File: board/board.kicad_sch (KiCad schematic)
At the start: 1 part, among them U1 ESP32-S3-DevKitC

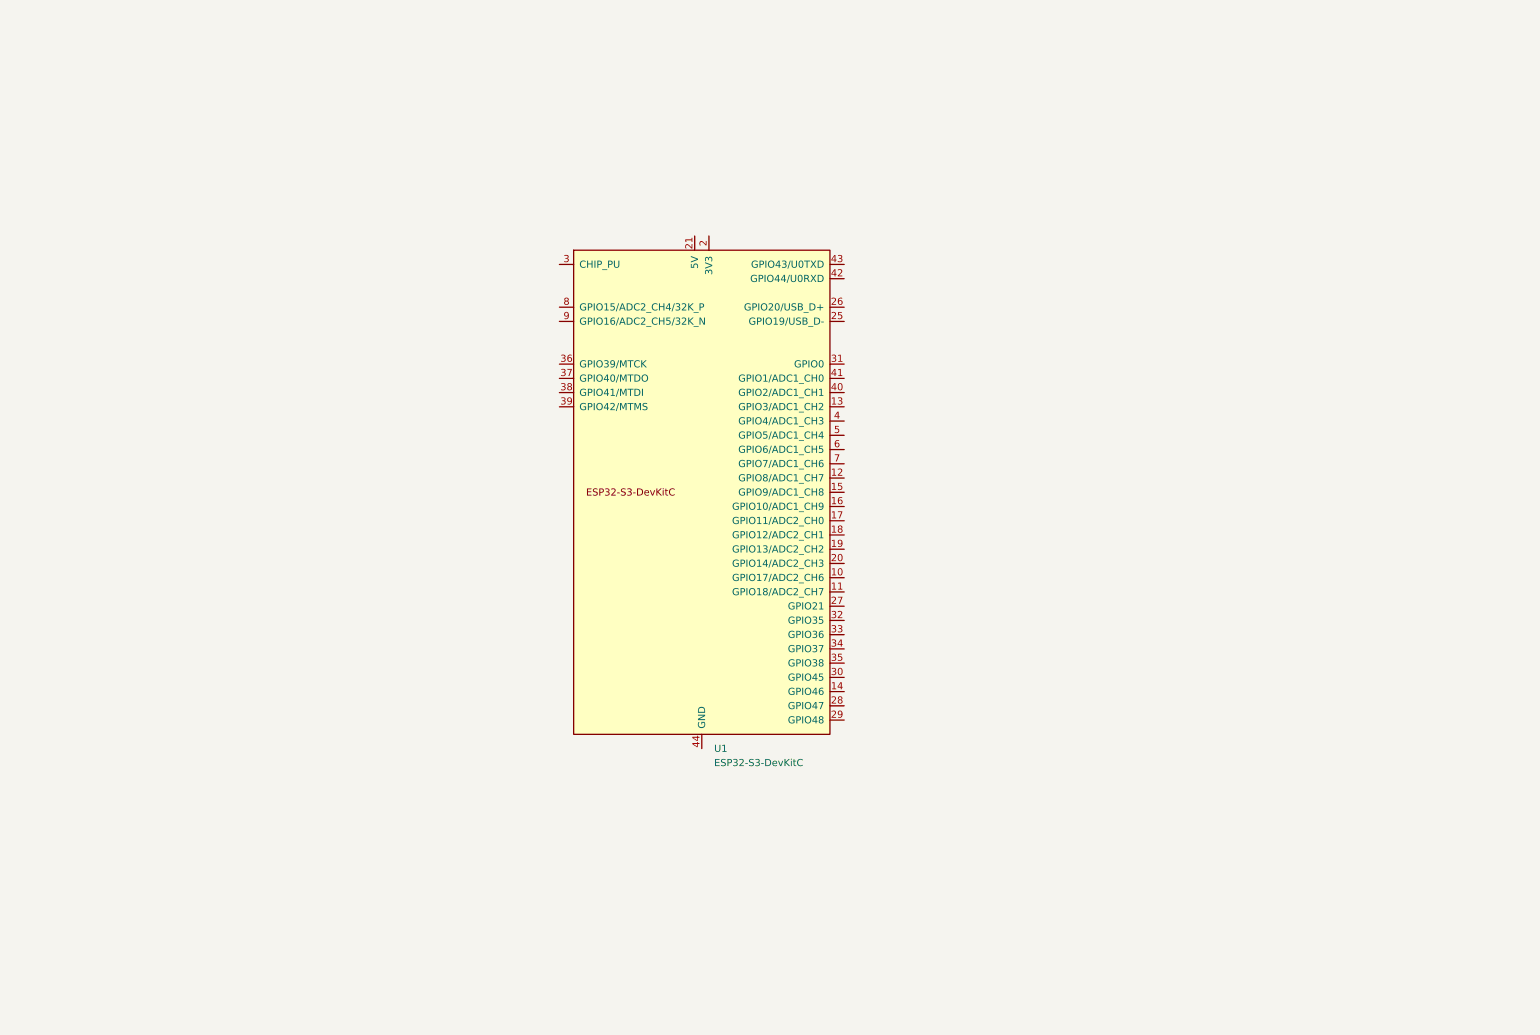
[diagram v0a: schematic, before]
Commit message: incremental changes
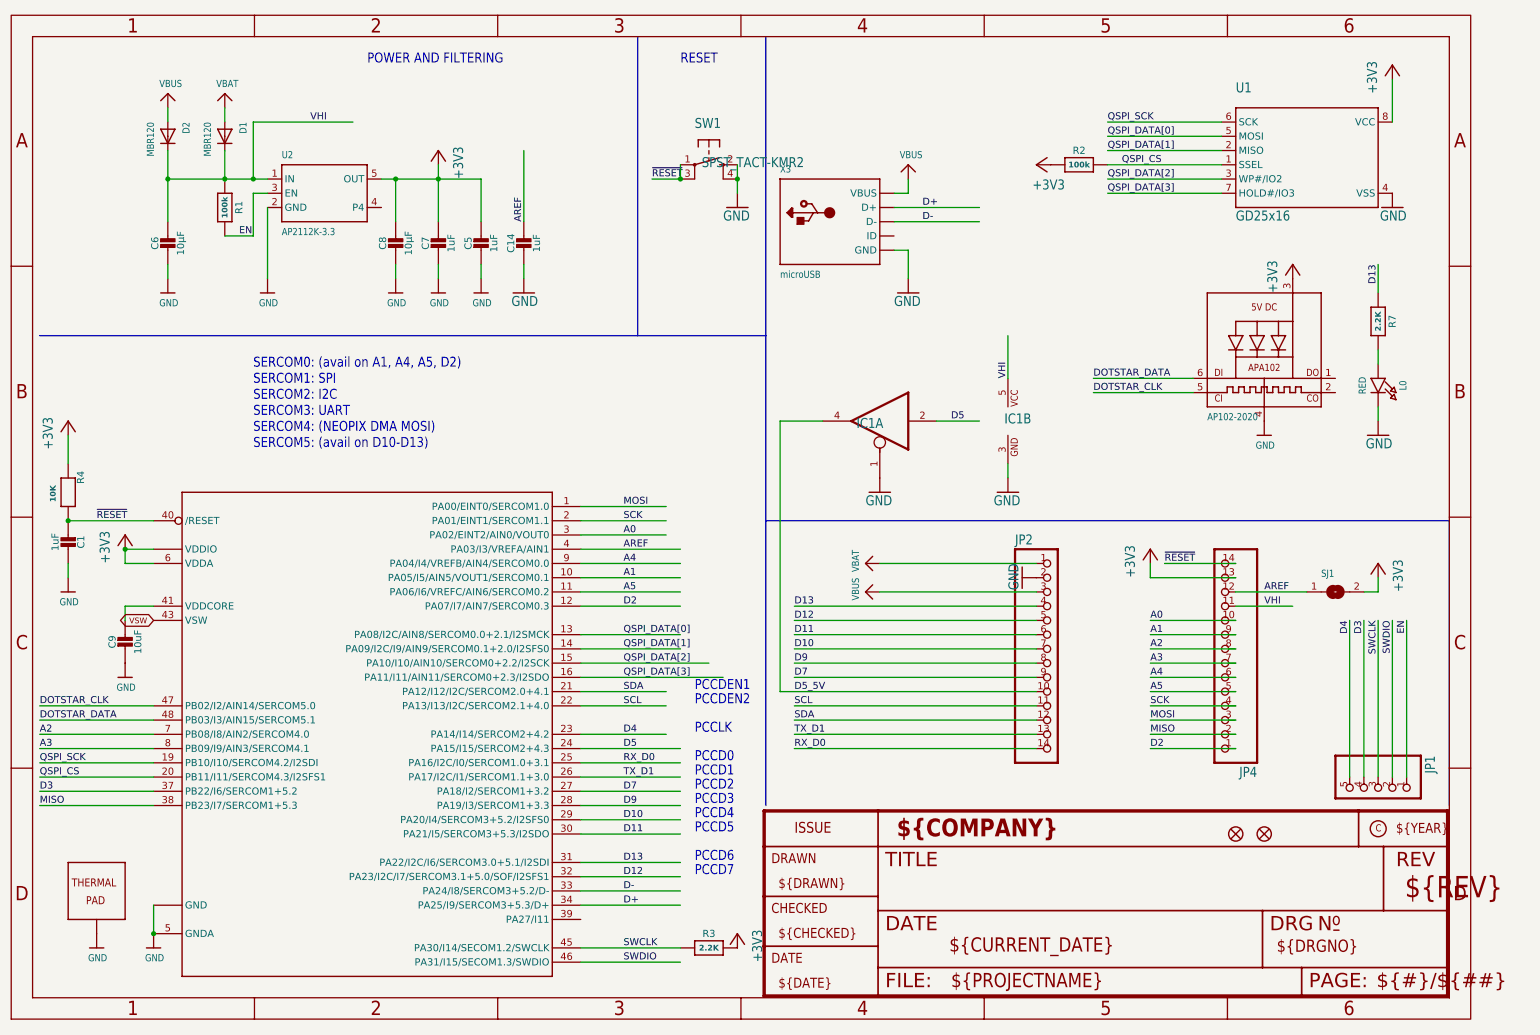
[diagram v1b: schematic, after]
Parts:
- removed U1: ESP32-S3-DevKitC, PCM_Espressif:ESP32-S3-DevKitC, symbol PCM_Espressif:ESP32-S3-DevKitC
- added C1: 1uF, board:_0603MP, symbol board-eagle-import:CAP_CERAMIC_0603MP
- added C14, C5, C7: 1uF, board:0603-NO, symbol board-eagle-import:CAP_CERAMIC0603_NO
- added C6, C8: 10µF, board:0805-NO, symbol board-eagle-import:CAP_CERAMIC0805-NOOUTLINE
- added C9: 10uF, board:_0805MP, symbol board-eagle-import:CAP_CERAMIC_0805MP
- added D1, D2: MBR120, board:SOD-123FL, symbol board-eagle-import:DIODE_SOD-123FL
- added IC1: 74HCT1G125DBV, board:SOT23-5, symbol board-eagle-import:741G125DBV
- added IC2: ATSAMD51G_TQFN48, board:TQFN48_7MM, symbol board-eagle-import:ATSAMD51G_TQFN48
- added JP1: HEADER-1X570MIL, board:1X05_ROUND_70, symbol board-eagle-import:HEADER-1X570MIL
- added JP2, JP4: HEADER-1X14, board:1X14_ROUND70, symbol board-eagle-import:HEADER-1X14
- added L0: RED, board:CHIPLED_0603_NOOUTLINE, symbol board-eagle-import:LED0603_NOOUTLINE
- added L2: AP102-2020, board:APA102_2020, symbol board-eagle-import:APA1022020
- added R1, R2: 100k, board:0603-NO, symbol board-eagle-import:RESISTOR_0603_NOOUT
- added R3: 2.2K, board:_0603MP, symbol board-eagle-import:RESISTOR_0603MP
- added R4: 10K, board:_0603MP, symbol board-eagle-import:RESISTOR_0603MP
- added R7: 2.2K, board:0603-NO, symbol board-eagle-import:RESISTOR_0603_NOOUT
- added SJ1: SOLDERJUMPERCLOSED, board:SOLDERJUMPER_CLOSEDWIRE, symbol board-eagle-import:SOLDERJUMPERCLOSED
- added SW1: SPST_TACT-KMR2, board:KMR2, symbol board-eagle-import:SPST_TACT-KMR2
- added U$34, U$35: FIDUCIAL_1MM, board:FIDUCIAL_1MM, symbol board-eagle-import:FIDUCIAL_1MM
- added U1: GD25x16, board:USON8, symbol board-eagle-import:SPIFLASH_8PINUX
- added U2: AP2112K-3.3, board:SOT23-5, symbol board-eagle-import:VREG_SOT23-5
- added X3: microUSB, board:4UCONN_20329_V2, symbol board-eagle-import:USB_MICRO_20329_V2
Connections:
- new net: L0.A, R7.2
- new net: C9.1, IC2.41 (VDDCORE)
- new net +3V3: C5.1, C7.1, C8.1, IC2.17 (VDDIO), IC2.36 (VDDIO), IC2.44 (VDDIO), IC2.6 (VDDA), JP4.13, L2.3 (VDD), R2.1, R3.2, R4.1, SJ1.2, U1.8 (VCC), U2.5 (OUT)
- new net A0: IC2.3 (PA02/EINT2/AIN0/VOUT0), JP4.10
- new net A1: IC2.10 (PA05/I5/AIN5/VOUT1/SERCOM0.1), JP4.9
- new net A2: IC2.7 (PB08/I8/AIN2/SERCOM4.0), JP4.8
- new net A3: IC2.8 (PB09/I9/AIN3/SERCOM4.1), JP4.7
- new net A4: IC2.9 (PA04/I4/VREFB/AIN4/SERCOM0.0), JP4.6
- new net A5: IC2.11 (PA06/I6/VREFC/AIN6/SERCOM0.2), JP4.5
- new net AREF: C14.1, IC2.4 (PA03/I3/VREFA/AIN1), JP4.12, SJ1.1
- new net D+: IC2.34 (PA25/I9/SERCOM3+5.3/D+), X3.D+
- new net D-: IC2.33 (PA24/I8/SERCOM3+5.2/D-), X3.D-
- new net D10: IC2.29 (PA20/I4/SERCOM3+5.2/I2SFS0), JP2.7
- new net D11: IC2.30 (PA21/I5/SERCOM3+5.3/I2SDO), JP2.6
- new net D12: IC2.32 (PA23/I2C/I7/SERCOM3.1+5.0/SOF/I2SFS1), JP2.5
- new net D13: IC2.31 (PA22/I2C/I6/SERCOM3.0+5.1/I2SDI), JP2.4, R7.1
- new net D2: IC2.12 (PA07/I7/AIN7/SERCOM0.3), JP4.1
- new net D3: IC2.37 (PB22/I6/SERCOM1+5.2), JP1.4
- new net D4: IC2.23 (PA14/I14/SERCOM2+4.2), JP1.5
- new net D5: IC1.2 (I), IC2.24 (PA15/I15/SERCOM2+4.3)
- new net D5_5V: IC1.4 (O), JP2.10
- new net D7: IC2.27 (PA18/I2/SERCOM1+3.2), JP2.9
- new net D9: IC2.28 (PA19/I3/SERCOM1+3.3), JP2.8
- new net DOTSTAR_CLK: IC2.47 (PB02/I2/AIN14/SERCOM5.0), L2.5 (CKI)
- new net DOTSTAR_DATA: IC2.48 (PB03/I3/AIN15/SERCOM5.1), L2.6 (DI)
- new net EN: JP1.1, R1.2, U2.3 (EN)
- new net GND: C1.1, C14.2, C5.2, C6.2, C7.2, C8.2, C9.2, IC1.1 (OE), IC1.3 (GND), IC2.18 (GND), IC2.35 (GND), IC2.42 (GND), IC2.5 (GNDA), IC2.THERMAL (TP), JP2.2, L0.C, L2.4 (GND), SW1.2 (S), SW1.4 (S1), U1.4 (VSS), U2.2 (GND), X3.BASE@1 (GND), X3.BASE@2 (GND), X3.GND, X3.SPRT@1 (GND), X3.SPRT@2 (GND), X3.SPRT@3 (GND), X3.SPRT@4 (GND)
- new net MISO: IC2.38 (PB23/I7/SERCOM1+5.3), JP4.2
- new net MOSI: IC2.1 (PA00/EINT0/SERCOM1.0), JP4.3
- new net QSPI_CS: IC2.20 (PB11/I11/SERCOM4.3/I2SFS1), R2.2, U1.1 (SSEL)
- new net QSPI_DATA[0]: IC2.13 (PA08/I2C/AIN8/SERCOM0.0+2.1/I2SMCK), U1.5 (MOSI)
- new net QSPI_DATA[1]: IC2.14 (PA09/I2C/I9/AIN9/SERCOM0.1+2.0/I2SFS0), U1.2 (MISO)
- new net QSPI_DATA[2]: IC2.15 (PA10/I10/AIN10/SERCOM0+2.2/I2SCK), U1.3 (WP#/IO2)
- new net QSPI_DATA[3]: IC2.16 (PA11/I11/AIN11/SERCOM0+2.3/I2SDO), U1.7 (HOLD#/IO3)
- new net QSPI_SCK: IC2.19 (PB10/I10/SERCOM4.2/I2SDI), U1.6 (SCK)
- new net RX_D0: IC2.25 (PA16/I2C/I0/SERCOM1.0+3.1), JP2.14
- new net SCK: IC2.2 (PA01/EINT1/SERCOM1.1), JP4.4
- new net SCL: IC2.22 (PA13/I13/I2C/SERCOM2.1+4.0), JP2.11
- new net SDA: IC2.21 (PA12/I12/I2C/SERCOM2.0+4.1), JP2.12
- new net SWCLK: IC2.45 (PA30/I14/SECOM1.2/SWCLK), JP1.3, R3.1
- new net SWDIO: IC2.46 (PA31/I15/SECOM1.3/SWDIO), JP1.2
- new net TX_D1: IC2.26 (PA17/I2C/I1/SERCOM1.1+3.0), JP2.13
- new net VBAT: D1.A, JP2.1
- new net VBUS: D2.A, JP2.3, X3.VBUS
- new net VHI: C6.1, D1.C, D2.C, IC1.5 (VCC), JP4.11, R1.1, U2.1 (IN)
- new net VSW: IC2.43 (VSW)
- new net ~{RESET}: C1.2, IC2.40 (/RESET), JP4.14, R4.2, SW1.1 (P), SW1.3 (P1)
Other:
- note added: "PCCD0"
- note added: "PCCD1"
- note added: "PCCD2"
- note added: "PCCD3"
- note added: "PCCD4"
- note added: "PCCD5"
- note added: "PCCD6"
- note added: "PCCD7"
- note added: "PCCDEN1"
- note added: "PCCDEN2"
- note added: "PCCLK"
- note added: "POWER AND FILTERING"
- note added: "RESET"
- note added: "SERCOM0: (avail on A1, A4, A5, D2) SERCOM1: SPI SERCOM2: I2C SERCOM3: UART SERCOM4: (NEOPIX DMA MOSI) SERCOM5: (avail on D10-D13)"
